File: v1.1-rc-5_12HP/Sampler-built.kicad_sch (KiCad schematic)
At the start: 248 parts, among them J10 Eurorack_Power_10pin_Unshroud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, J11 3.5mm_Mono_Switched, J12 3.5mm_Mono_Switched, J13 3.5mm_Mono_Switched, J14 3.5mm_Mono_Switched, J15 3.5mm_Mono_Switched, J16 3.5mm_Mono_Switched, J17 3.5mm_Mono_Switched, J2 3.5mm_Mono_Switched, J3 Conn_01x04, J4 Conn_02x04, J6 3.5mm_Mono_Switched, J7 3.5mm_Mono_Switched, J8 3.5mm_Mono_Switched, J9 3.5mm_Mono_Switched, Q11 Si2347, Q12 Si2318, U1 TL072H, U10 TL072H, U11 TL072H, U12 TL072H, U13 AP62200WU-7, U14 TL072H, U15 TL072H, U16 TL072H, U18 STS SD card w/adaptor, U2 STM32F746IE, U3 TL072H, U4 SDRAM_IS42S16400J-6BLI-TR, U5 TL072H, U6 NCP51460SN33, U8 TL072H, U9 PCM3060PW, Y1 16MHz_18pF_FA238

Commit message: Changed 16v 100nf caps to be 50v and apear on same BOM line
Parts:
- C1, C10, C11, C12, C13, C14, C15, C16, C17, C18, C20, C25, C26, C27, C28, C29, C3, C30, C31, C32, C33, C36, C39, C41, C42, C45, C47, C50, C53, C54, C58, C6, C65, C66, C7, C79, C83, C9: Alt JLCPCB ID (none) -> C77020; JLCPCB ID C1525 -> C307331; Manufacturer 2 Yageo -> (none); Part Number GCM155R71C104KA55D -> GRM155R71H104KE14D; Part Number 2 CC0402KRX7R7BB104 -> (none); Specifications 0.1uF, Min. 16V 10%, X7R or X5R or similar -> 0.1uF, Min. 50V 10%, X7R or X5R or similar

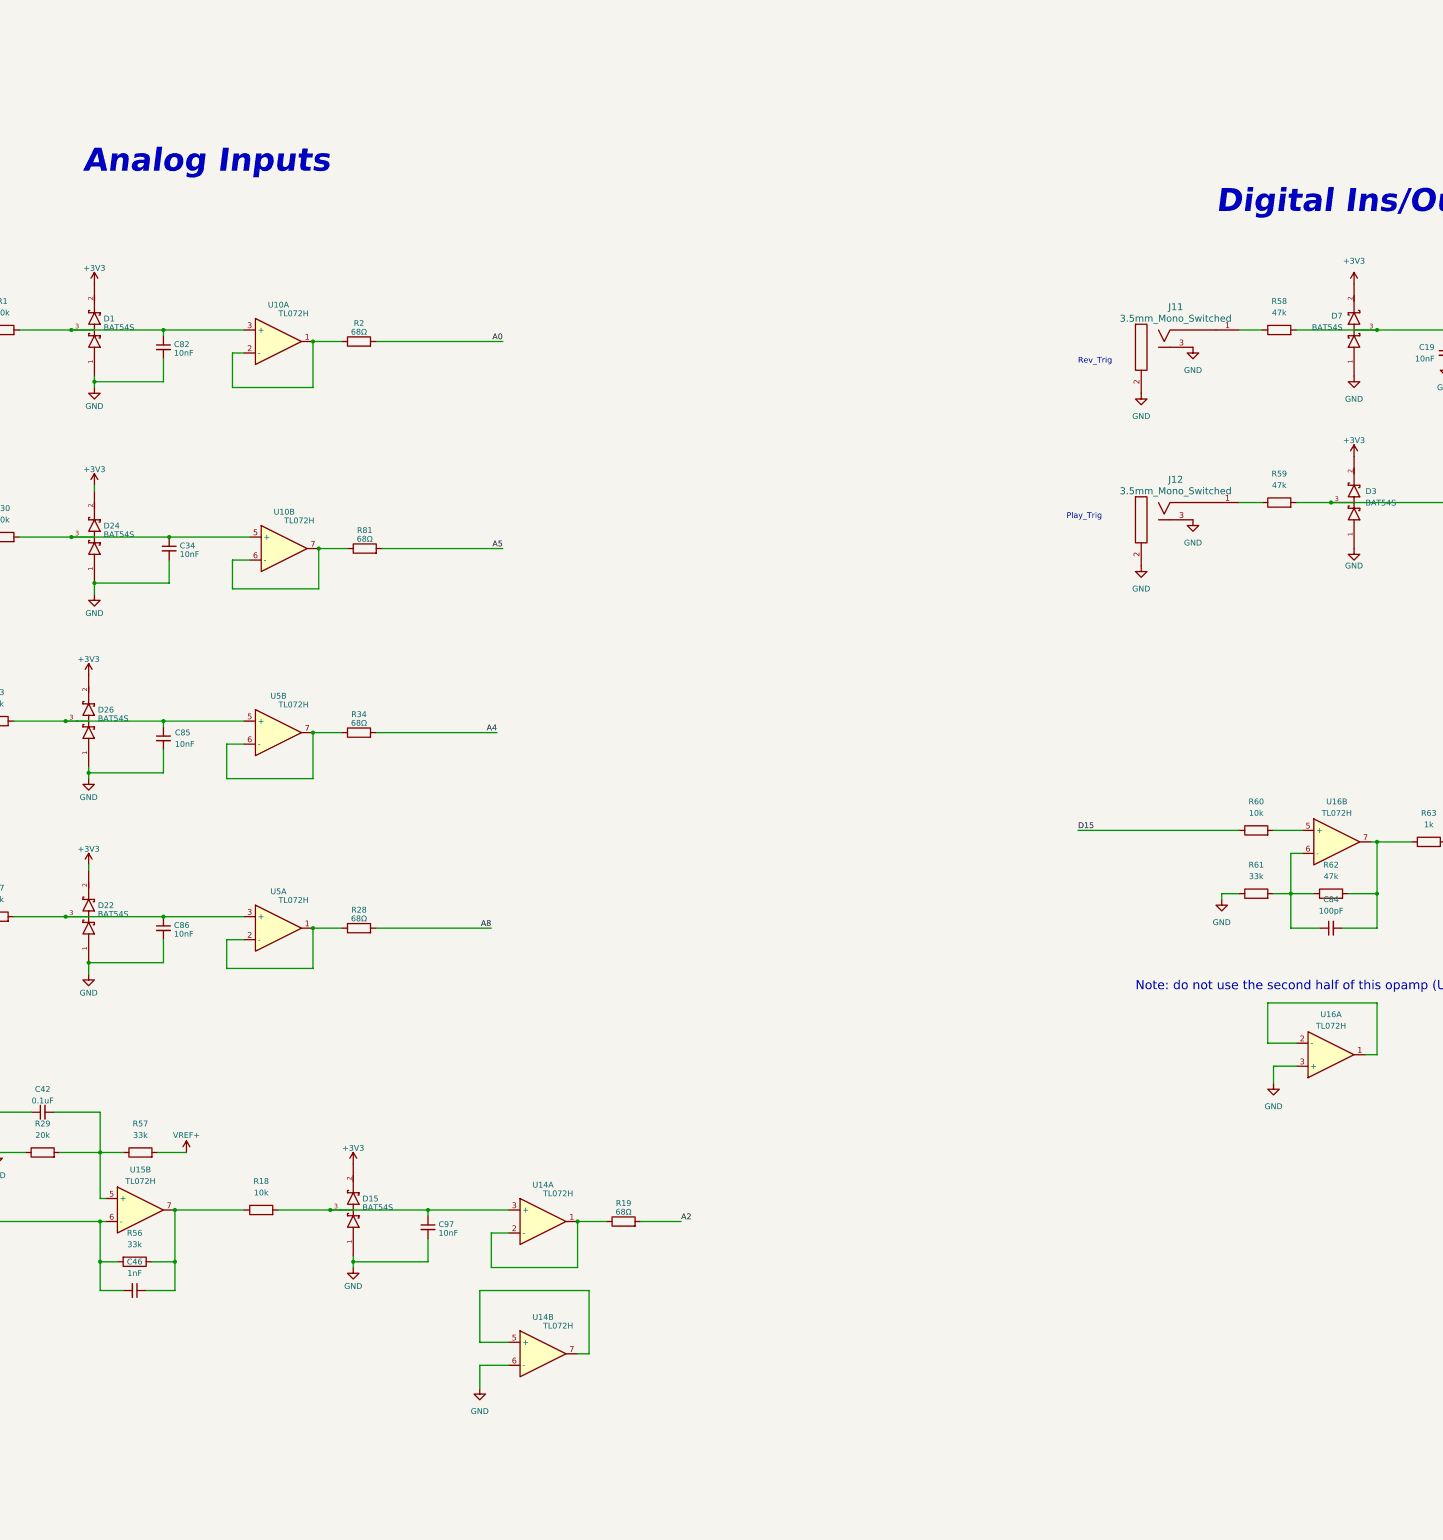
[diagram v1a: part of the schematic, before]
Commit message: Generated production files and submitted project
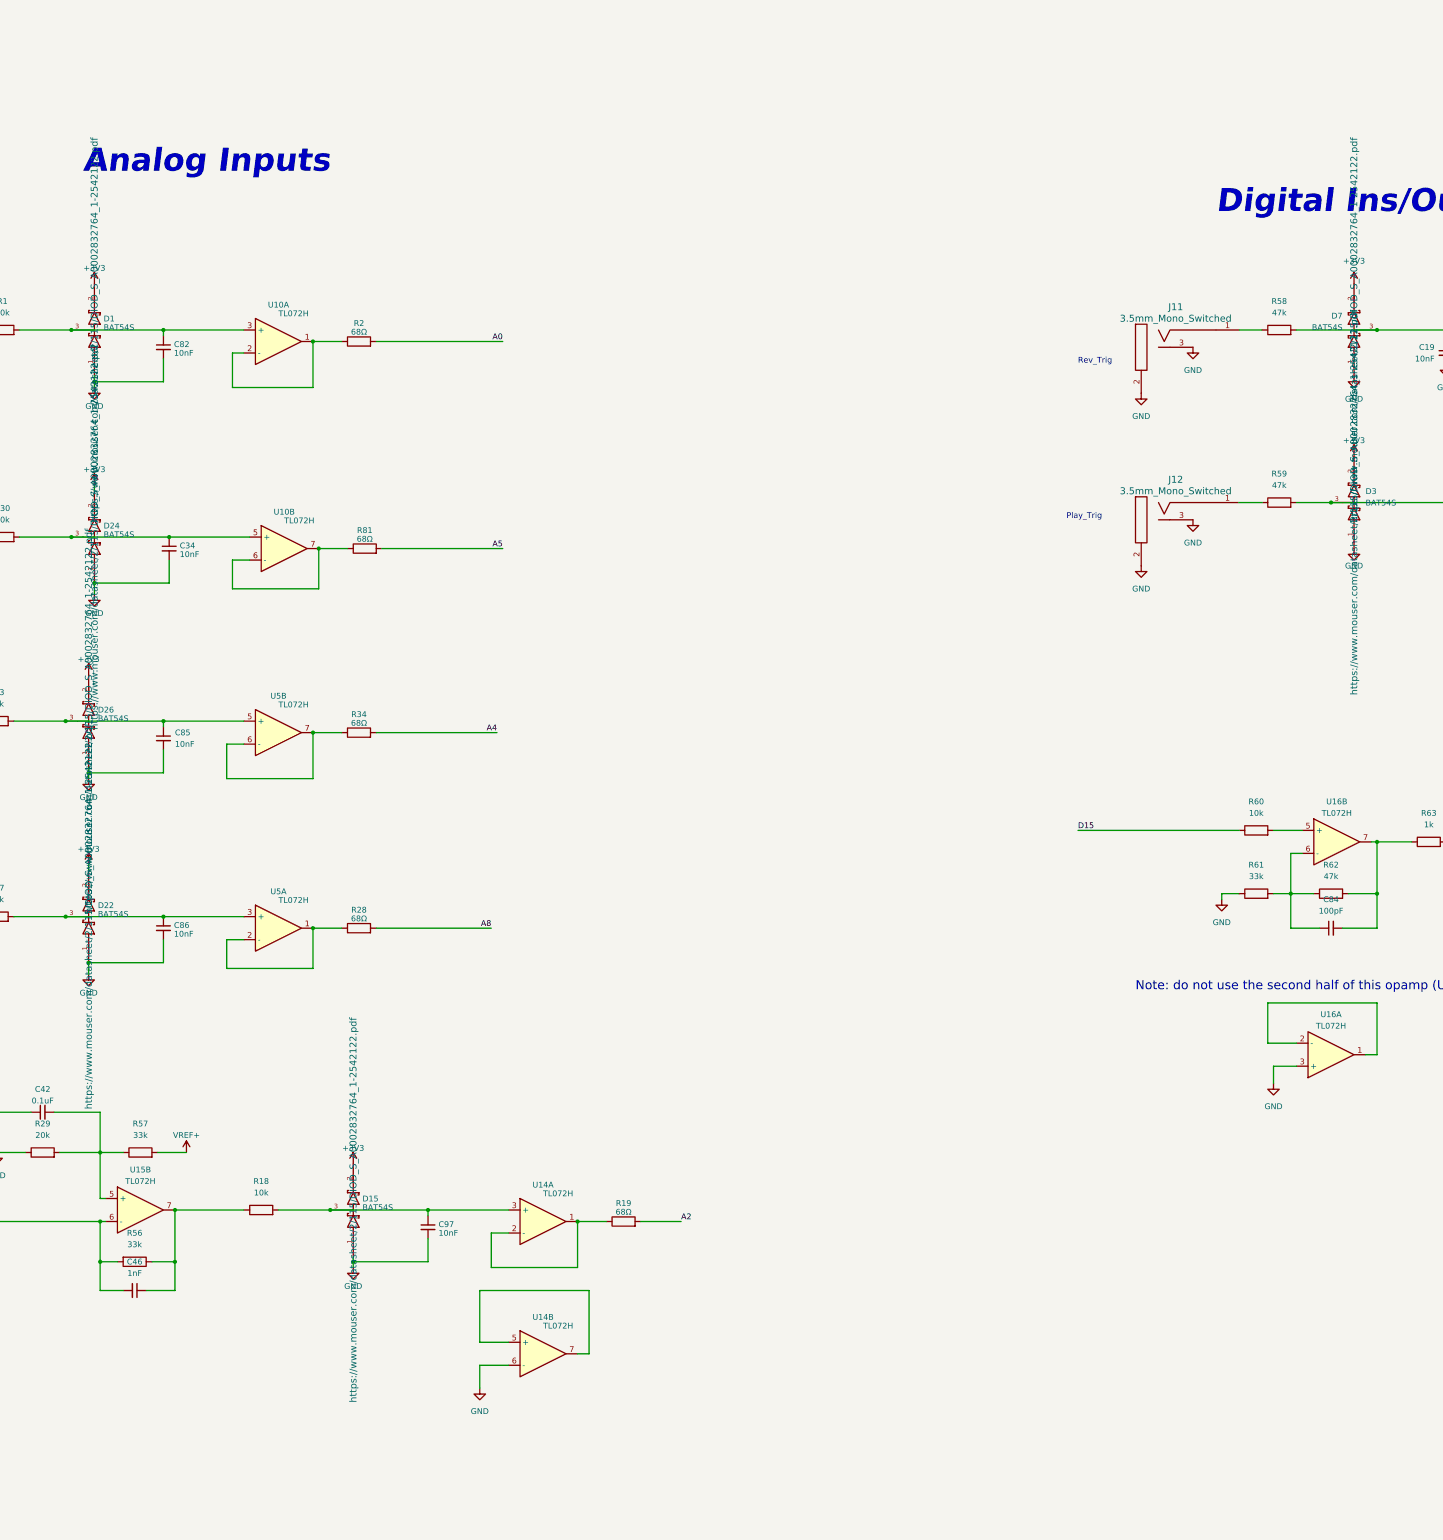
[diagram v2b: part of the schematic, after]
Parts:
- JP11, JP2, JP3, JP4: footprint 4ms_SolderJumper:JUMPER_SMD_1x2_tiny_shorted -> 4ms_SolderJumper:Net_Tie_0.16mm_6mil
